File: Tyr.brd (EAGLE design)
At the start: 152.4 x 115.6 mm, 206 parts, among them J1 TYR_TYR_DISPLAY, Q1 DTC123J, SW1 BUTTON, U1 MCP1700T, U2 CONTROLLER_PRTR5V0U2X, U3 STM32F303CC, U4 MB85RC256V, U6 TYR_TPS2552, X1 CONTROLLER_USB-C-12PUSB-C-12P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, Y1 8Mhz

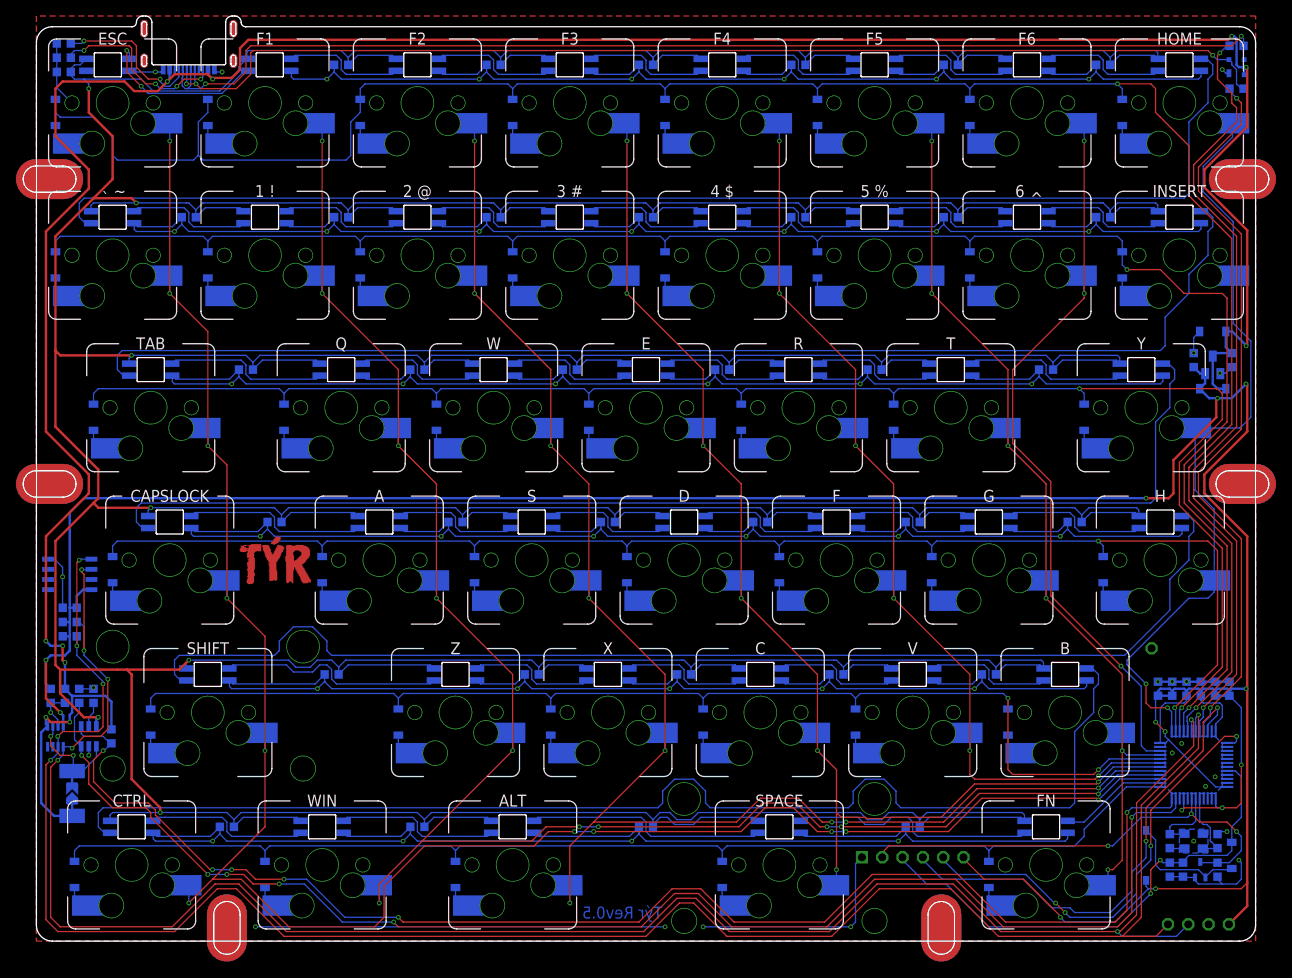
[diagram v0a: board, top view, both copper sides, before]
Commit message: Y branching
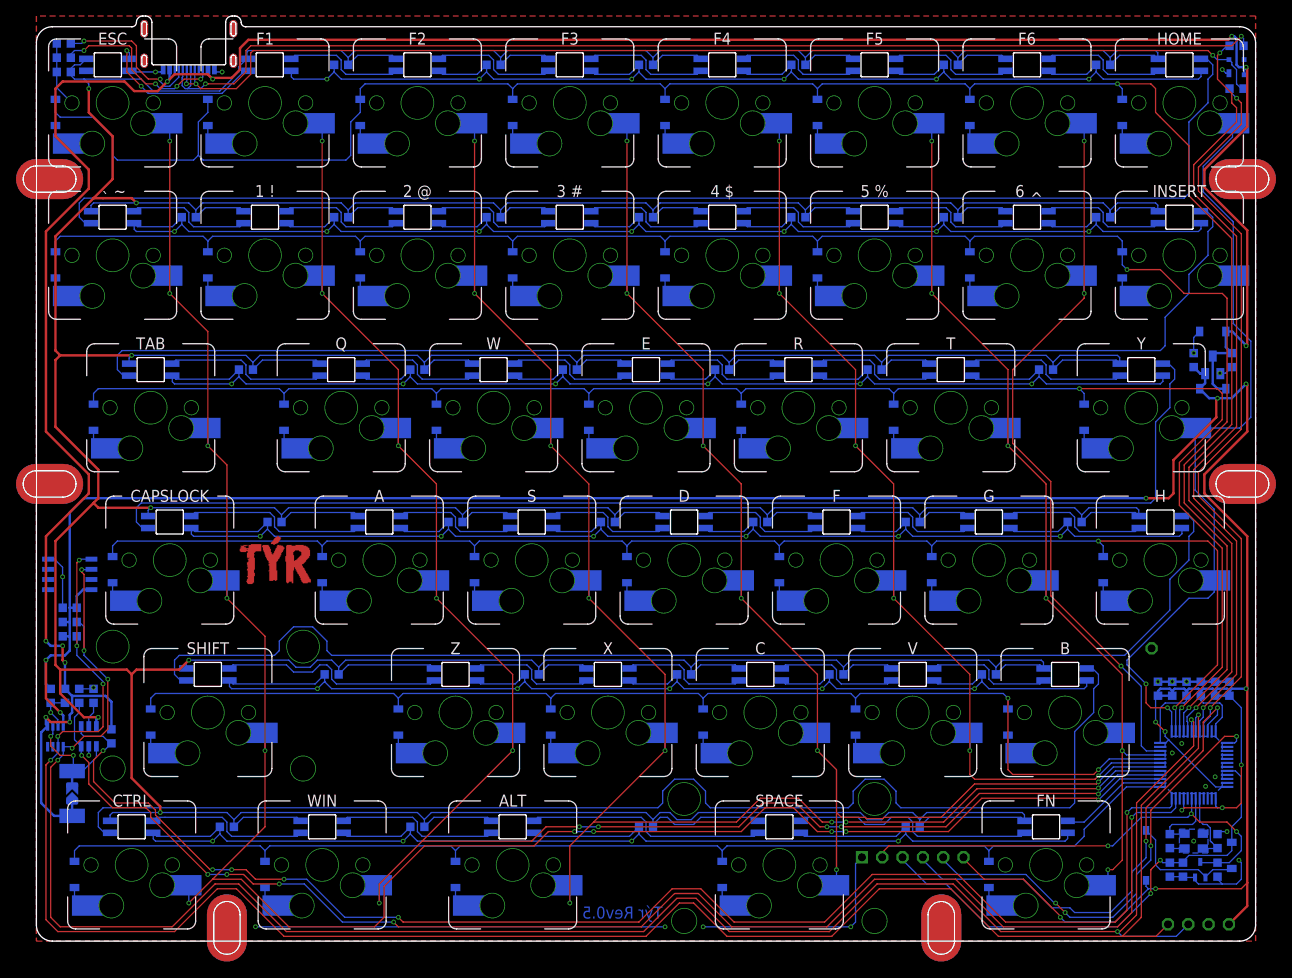
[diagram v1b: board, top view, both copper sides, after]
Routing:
- net LED_VCC: track 1250.6 -> 1226.3 mm
